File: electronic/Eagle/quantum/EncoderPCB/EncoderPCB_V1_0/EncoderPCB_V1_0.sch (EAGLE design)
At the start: 15 parts, among them IC1 STM32F031K6T7

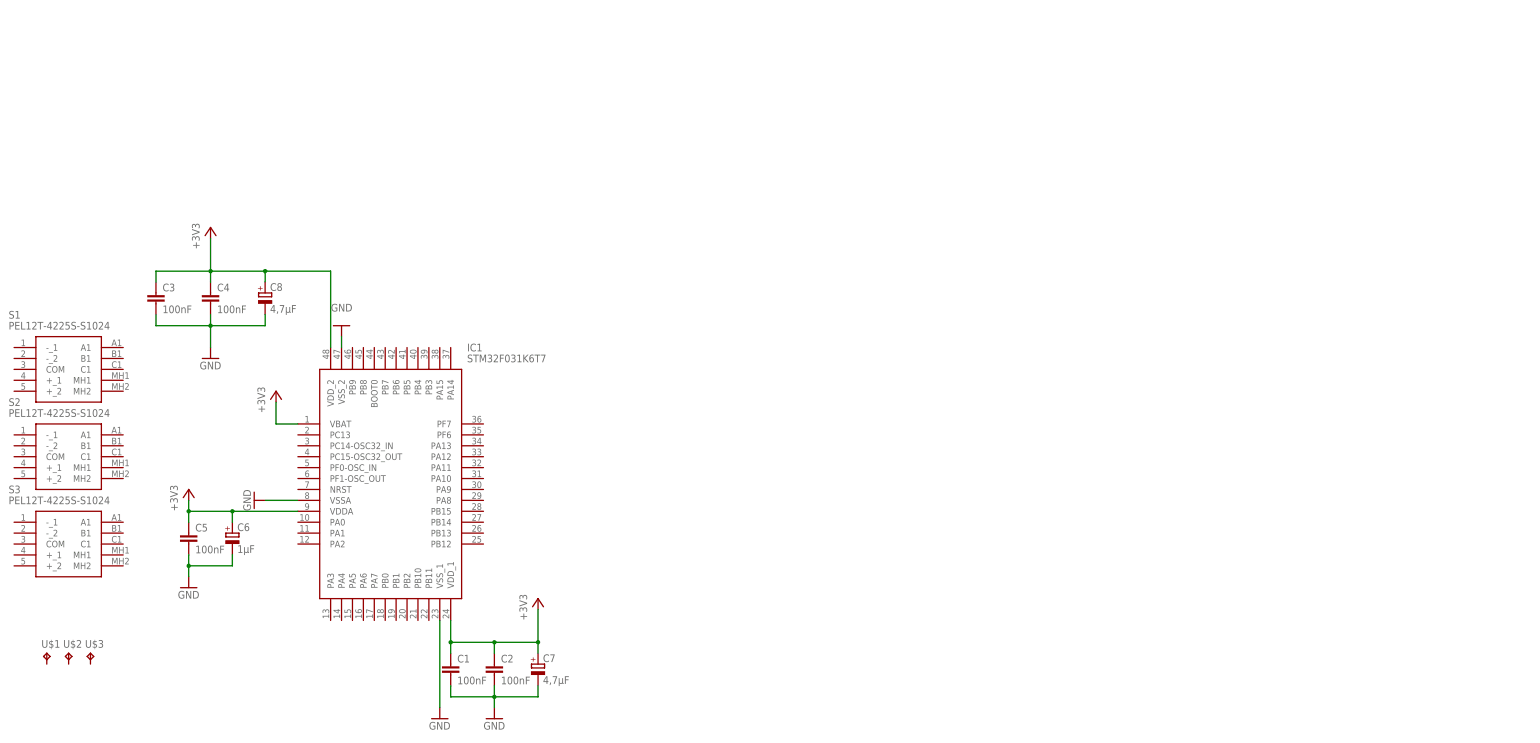
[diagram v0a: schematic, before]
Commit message: Encoder PCB_V1_0 fertiggestellt
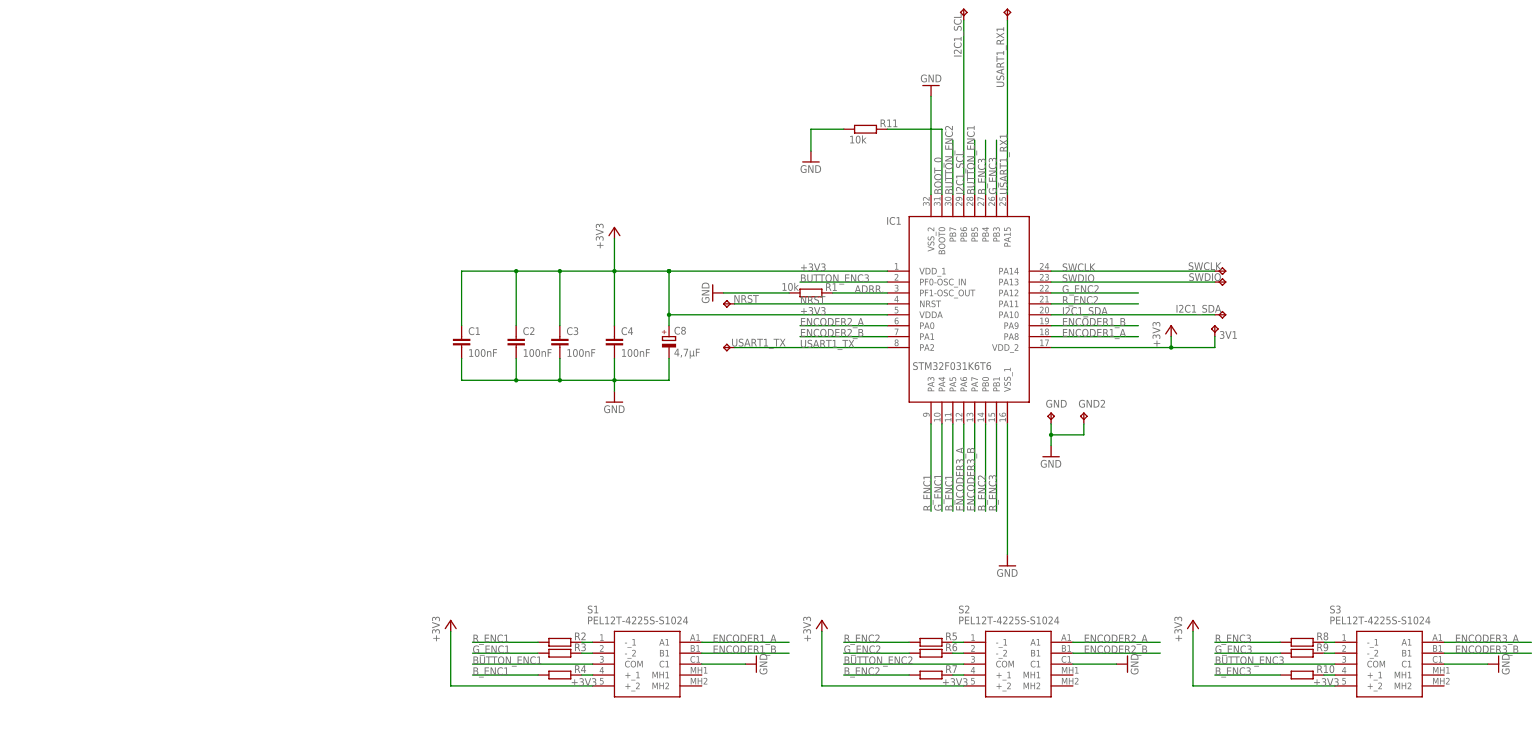
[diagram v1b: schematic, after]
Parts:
- removed C5: 100nF, C_Sager_Bibliothek:CAPACITOR"
- removed C6: 1µF, C_Sager_Bibliothek:SMD_ELCTROLYTIC
- removed C7: 4,7µF, C_Sager_Bibliothek:SMD_ELCTROLYTIC
- removed U$1, U$2, U$3: TPTHT, C_Sager_Bibliothek:TPTHT
- added 3V1, GND, GND2, I2C1_SCL, I2C1_SDA, NRST, SWCLK, SWDIO, USART1_RX1, USART1_TX: TPTHT, C_Sager_Bibliothek:TPTHT
- added R1, R11: 10k, C_Sager_Bibliothek:RESISTOR"
- added R10, R2, R3, R4, R5, R6, R7, R8, R9: (no value), C_Sager_Bibliothek:RESISTOR"
- IC1: value STM32F031K6T7 -> STM32F031K6T6; device C_Sager_Bibliothek:STM32F031K6T7 -> C_Sager_Bibliothek:STM32F031K6T6
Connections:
- new net ADRR.: IC1.PF1-OSC_OUT, R1.2
- new net BOOT_0: IC1.BOOT0, R11.2
- new net BUTTON_ENC1: IC1.PB5, S1.COM
- new net BUTTON_ENC2: IC1.PB7, S2.COM
- new net BUTTON_ENC3: IC1.PF0-OSC_IN, S3.COM
- new net B_ENC1: IC1.PA5, R4.1
- new net B_ENC2: IC1.PB0, R7.1
- new net B_ENC3: IC1.PB4, R10.1
- new net ENCODER1_A: IC1.PA8, S1.A1
- new net ENCODER1_B: IC1.PA9, S1.B1
- new net ENCODER2_A: IC1.PA0, S2.A1
- new net ENCODER2_B: IC1.PA1, S2.B1
- new net ENCODER3_A: IC1.PA6, S3.A1
- new net ENCODER3_B: IC1.PA7, S3.B1
- new net G_ENC1: IC1.PA4, R3.1
- new net G_ENC2: IC1.PA12, R6.1
- new net G_ENC3: IC1.PB3, R9.1
- new net I2C1_SCL: I2C1_SCL.TP, IC1.PB6
- new net I2C1_SDA: I2C1_SDA.TP, IC1.PA10
- new net N$10: R3.2, S1.-_2
- new net N$11: R5.2, S2.-_1
- new net N$12: R4.2, S1.+_1
- new net N$13: R6.2, S2.-_2
- new net N$14: R7.2, S2.+_1
- new net N$15: R8.2, S3.-_1
- new net N$16: R9.2, S3.-_2
- new net N$17: R10.2, S3.+_1
- new net N$9: R2.2, S1.-_1
- new net NRST: IC1.NRST, NRST.TP
- new net R_ENC1: IC1.PA3, R2.1
- new net R_ENC2: IC1.PA11, R5.1
- new net R_ENC3: IC1.PB1, R8.1
- new net SWCLK: IC1.PA14, SWCLK.TP
- new net SWDIO: IC1.PA13, SWDIO.TP
- new net USART1_RX1: IC1.PA15, USART1_RX1.TP
- new net USART1_TX: IC1.PA2, USART1_TX.TP
- net +3V3: now also 3V1.TP, S1.+_2, S2.+_2, S3.+_2; no longer C5.1, C6.+, C7.+, IC1.VBAT
- net GND: now also GND.TP, GND2.TP, R1.1, R11.1, S1.C1, S2.C1, S3.C1; no longer C5.2, C6.-, C7.-, IC1.VSSA
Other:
- moved on the sheet: C1, C2, C3, C4, C8, S1, S2, S3
